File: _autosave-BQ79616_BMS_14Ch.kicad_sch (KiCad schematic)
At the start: 164 parts, among them J1 Conn_Therm, J2 Conn_02x10_Odd_Even, J3 Conn_02x10_Odd_Even, J4 BMS_A_OUT, J5 BMS_A_IN, Q1 MMBT5551

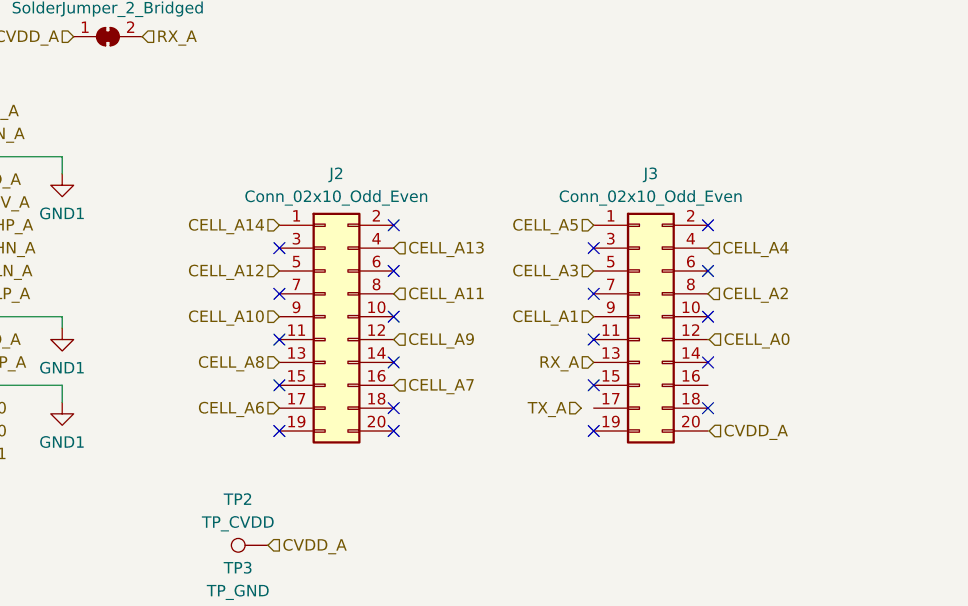
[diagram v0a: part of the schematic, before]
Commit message: Finish positioning of all components Ver1ST
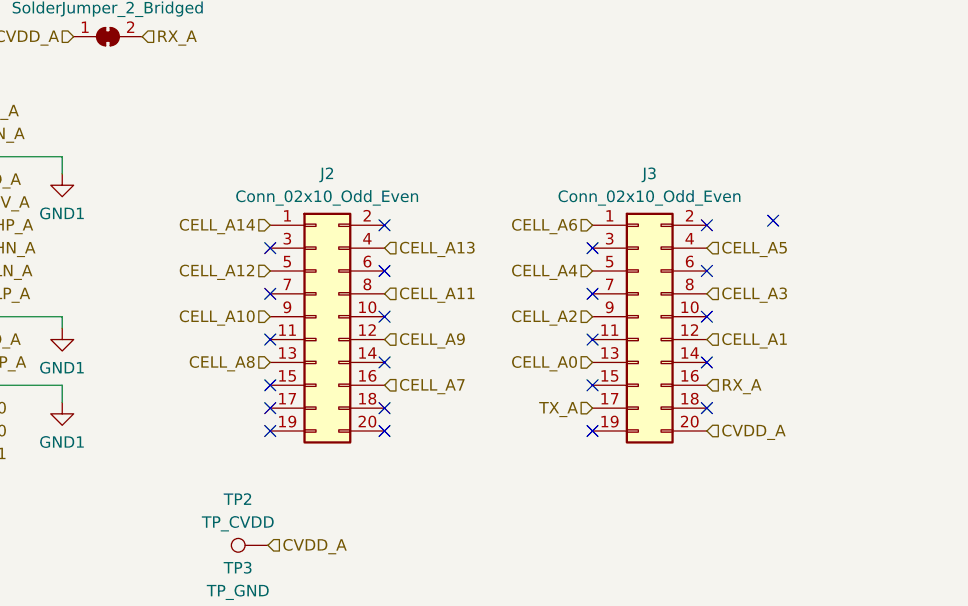
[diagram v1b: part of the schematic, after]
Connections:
- net CELL_A1: now also J3.12 (Pin_12); no longer J3.9 (Pin_9)
- net CELL_A2: now also J3.9 (Pin_9); no longer J3.8 (Pin_8)
- net CELL_A3: now also J3.8 (Pin_8); no longer J3.5 (Pin_5)
- net CELL_A4: now also J3.5 (Pin_5); no longer J3.4 (Pin_4)
- net CELL_A5: now also J3.4 (Pin_4); no longer J3.1 (Pin_1)
- net CELL_A6: now also J3.1 (Pin_1); no longer J2.17 (Pin_17)
- net CVDD_A: now also J3.20 (Pin_20)
- net GND1: now also J3.13 (Pin_13); no longer J3.12 (Pin_12)
- net RX_A: now also J3.16 (Pin_16); no longer J3.13 (Pin_13)
- net TX_A: now also J3.17 (Pin_17)
- no-connect marks 30 -> 32
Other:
- moved on the sheet: J2
